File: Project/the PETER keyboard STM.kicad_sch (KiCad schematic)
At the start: 140 parts, among them J3 USB_C_Receptacle_USB2.0, SW1 RotaryEncoder_Switch, SW12 RotaryEncoder_Switch, SW3 SKQGABE010, U2 STM32F072C8Tx, U3 XC6206PxxxMR-Regulator_Linear, U4 USBLC6-2SC6

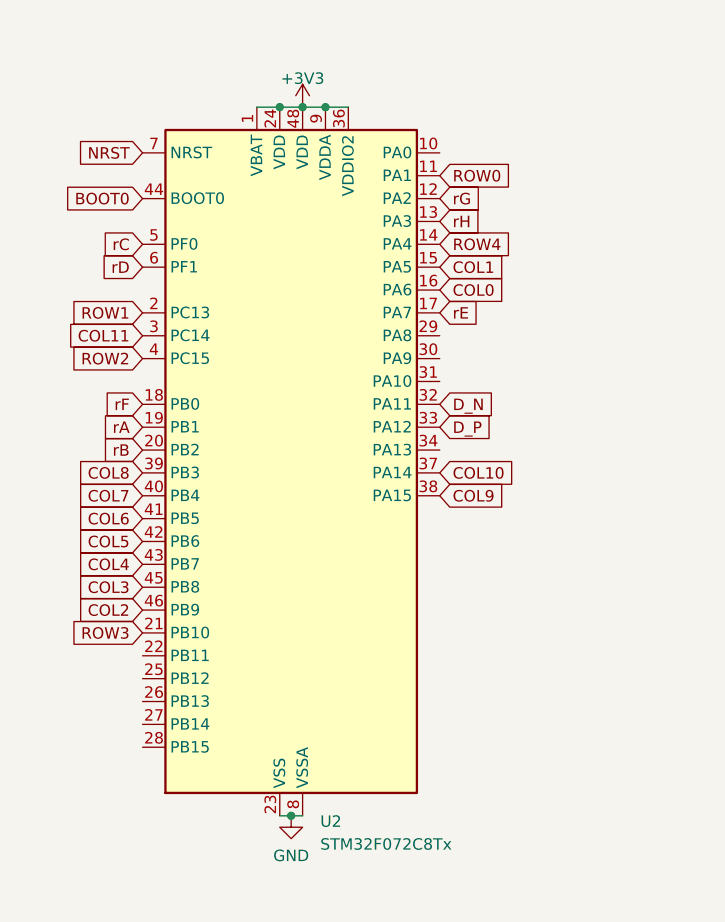
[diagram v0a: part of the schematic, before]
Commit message: stm revision
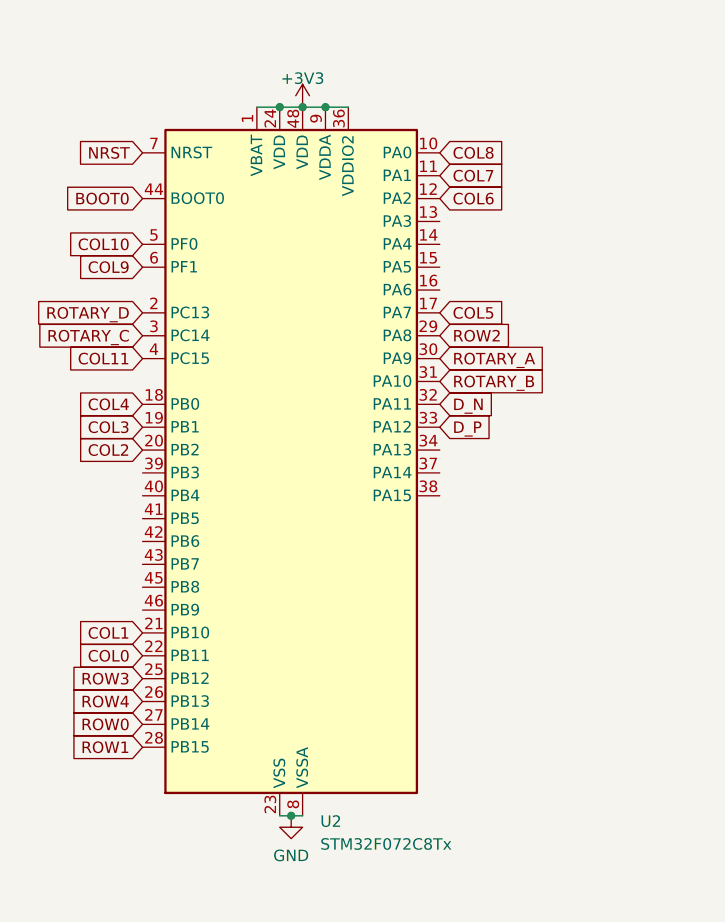
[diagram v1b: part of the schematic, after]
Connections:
- net  ROW3 is gone; now on net ROW3: D37.1 (K), D38.1 (K), D39.1 (K), D40.1 (K), D41.1 (K), D42.1 (K), D43.1 (K), D44.1 (K), D45.1 (K), D46.1 (K), D47.1 (K), D48.1 (K)
- net rA is gone; now on net COL3: U2.19 (PB1)
- net rB is gone; now on net COL2: U2.20 (PB2)
- net rC is gone; now on net COL10: U2.5 (PF0)
- net rD is gone; now on net COL9: U2.6 (PF1)
- net rE is gone; now on net COL5: U2.17 (PA7)
- net rF is gone; now on net COL4: U2.18 (PB0)
- net rG is gone; now on net COL6: U2.12 (PA2)
- net COL0: now also U2.22 (PB11); no longer U2.16 (PA6)
- net COL1: now also U2.21 (PB10); no longer U2.15 (PA5)
- net COL10: no longer U2.37 (PA14)
- net COL11: now also U2.4 (PC15); no longer U2.3 (PC14)
- net COL2: no longer U2.46 (PB9)
- net COL3: no longer U2.45 (PB8)
- net COL4: no longer U2.43 (PB7)
- net COL5: no longer U2.42 (PB6)
- net COL6: no longer U2.41 (PB5)
- net COL7: now also U2.11 (PA1); no longer U2.40 (PB4)
- net COL8: now also U2.10 (PA0); no longer U2.39 (PB3)
- net COL9: no longer U2.38 (PA15)
- net ROTARY_A: now also U2.30 (PA9)
- net ROTARY_B: now also U2.31 (PA10)
- net ROTARY_C: now also U2.3 (PC14)
- net ROTARY_D: now also U2.2 (PC13)
- net ROW0: now also U2.27 (PB14); no longer U2.11 (PA1)
- net ROW1: now also U2.28 (PB15); no longer U2.2 (PC13)
- net ROW2: now also U2.29 (PA8); no longer U2.4 (PC15)
- net ROW3: now also U2.25 (PB12); no longer U2.21 (PB10)
- net ROW4: now also U2.26 (PB13); no longer U2.14 (PA4)
- net rH: no longer names the net of U2.13 (PA3)
